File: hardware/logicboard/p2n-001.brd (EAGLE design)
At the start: 91 x 90 mm, 59 parts, among them IC1 74ALS05N, IC2 4066N, J1 MKR, J10 1-Wire, J2 GPIO, J3 Vcc, J4** RLY2, J5 SPI, J6 LED, J7 DIN5, J8 DIN5, J9 DIN5, K1 G5V1, T1 2SC1815

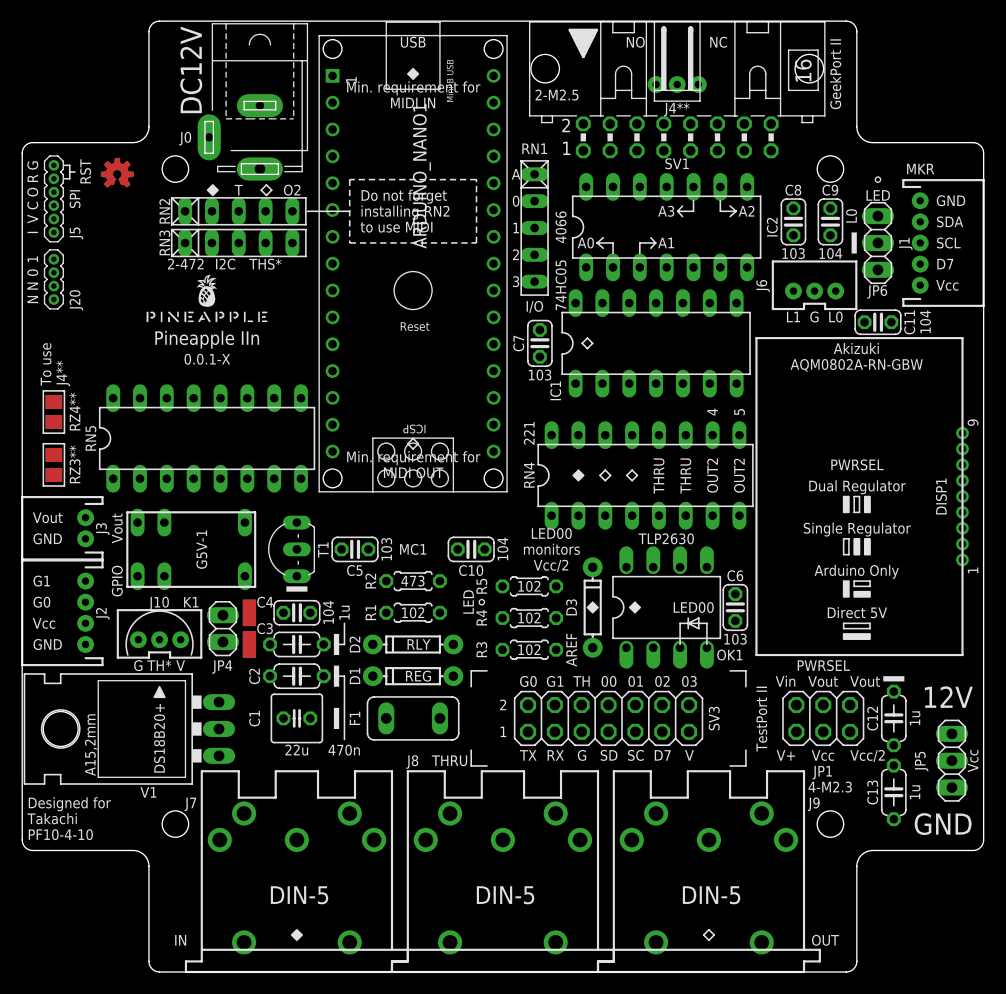
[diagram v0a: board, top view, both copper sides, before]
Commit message: First try.
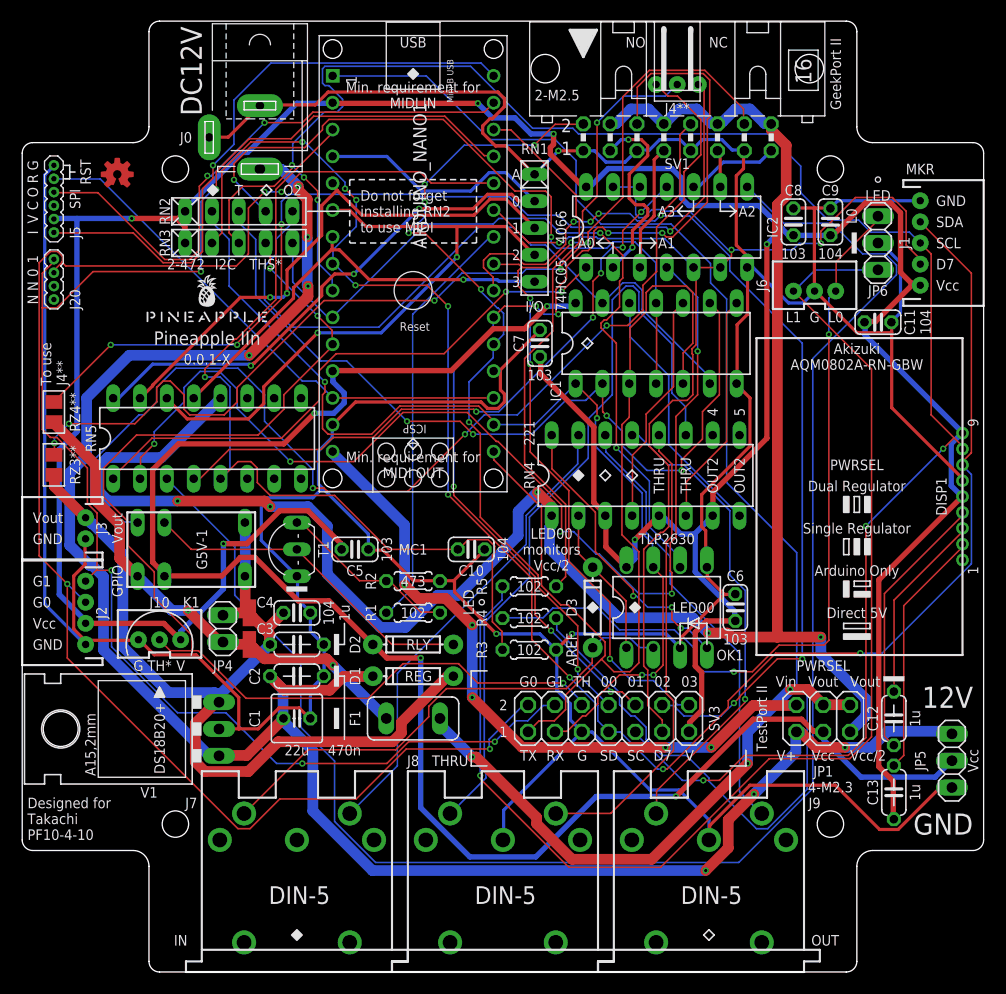
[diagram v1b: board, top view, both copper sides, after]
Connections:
- net VCC: no longer RN4.3, RN4.5, RN4.7
- net VDD: now also RN4.3, RN4.5, RN4.7
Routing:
- net GND: track 0.00 -> 450.4 mm, vias 0 -> 3
- net VDD: track 0.00 -> 333.8 mm, vias 0 -> 6
- net VCC/2: track 0.00 -> 187.5 mm, vias 0 -> 5
- net V+: track 0.00 -> 186.2 mm, vias 0 -> 7
- net SCL: track 0.00 -> 181.9 mm, vias 0 -> 6
- net SDA: track 0.00 -> 169.2 mm, vias 0 -> 9
- net VCC: track 0.00 -> 164.5 mm, vias 0 -> 4
- net N$3: track 0.00 -> 158.8 mm
- net GPIO0: track 0.00 -> 149.2 mm, vias 0 -> 4
- net GPIO1: track 0.00 -> 148.0 mm, vias 0 -> 5
- net LED0: track 0.00 -> 134.5 mm
- net LED1A: track 0.00 -> 118.8 mm, vias 0 -> 1
- net D7GATE: track 0.00 -> 117.7 mm, vias 0 -> 3
- net THS: track 0.00 -> 105.9 mm, vias 0 -> 3
- net N$2: track 0.00 -> 105.8 mm, vias 0 -> 5
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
